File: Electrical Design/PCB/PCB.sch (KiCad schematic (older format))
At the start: 59 parts, among them J1 Conn_02x03_Odd_Even, J2 10118193-0001LF, M1 Camera_Servo, M2 Release_Servo, Q1 LED_MOS, Q2 CAMERA_MOS, Q3 RELEASE_MOS, Q4 BUZZER_MOS, U1 ADP3338AKCZ-5-R7, U10 Adafruit_Cam, U2 BNO080, U3 ADP3338AKCZ-3.3-R7, U4 PCF8523T_1_118, U5 MS560702BA03-50, U6 SS495A, U7 Adafruit_746, U8 Openlog, U9 ATxmega128A4U-AU

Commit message: Fix Connector
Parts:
- J1: footprint Connector:Tag-Connect_TC2030-IDC-FP_2x03_P1.27mm_Vertical -> Connectors:2X3
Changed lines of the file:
@@
 F 0 "J1" H 1200 4600 50  0000 C CNN
 F 1 "Conn_02x03_Odd_Even" H 1200 4500 50  0000 C CNN
-F 2 "Connector:Tag-Connect_TC2030-IDC-FP_2x03_P1.27mm_Vertical" H 1150 4250 50  0001 C CNN
+F 2 "Connectors:2X3" H 1150 4250 50  0001 C CNN
 F 3 "~" H 1150 4250 50  0001 C CNN
 	1    1150 4250

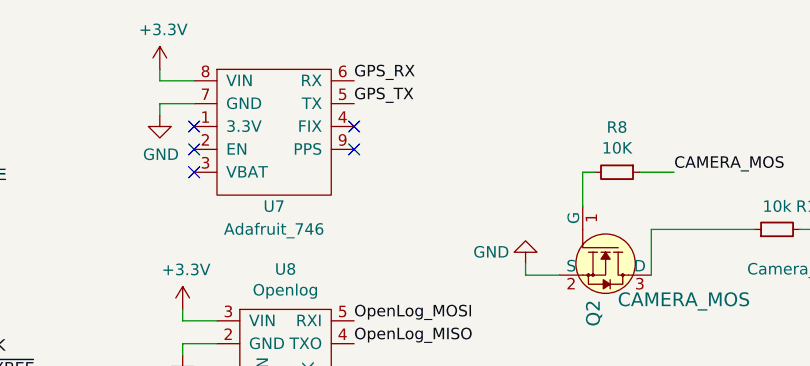
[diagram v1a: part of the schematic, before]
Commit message: m
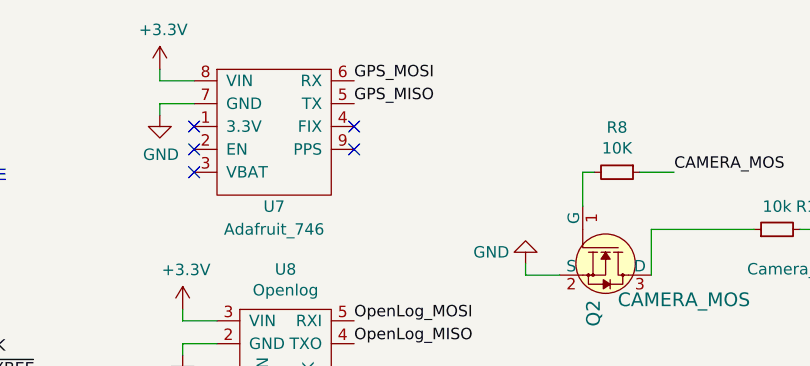
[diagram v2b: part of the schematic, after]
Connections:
- net GPS_RX is gone; now on net GPS_MOSI: U7.6 (RX)
- net GPS_TX is gone; now on net GPS_MISO: U7.5 (TX)
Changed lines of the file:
@@
 $EndComp
 Text Label 7200 800  0    50   ~ 0
-GPS_TX
+GPS_MISO
 Text Label 7200 700  0    50   ~ 0
-GPS_RX
+GPS_MOSI
 Text Label 8950 5150 2    50   ~ 0
 GPS_MISO
